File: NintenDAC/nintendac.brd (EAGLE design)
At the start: 42 x 42 mm, 36 parts, among them IC2 REG1117, U1 STM32F10XRXT6, X1 USB-MICROB

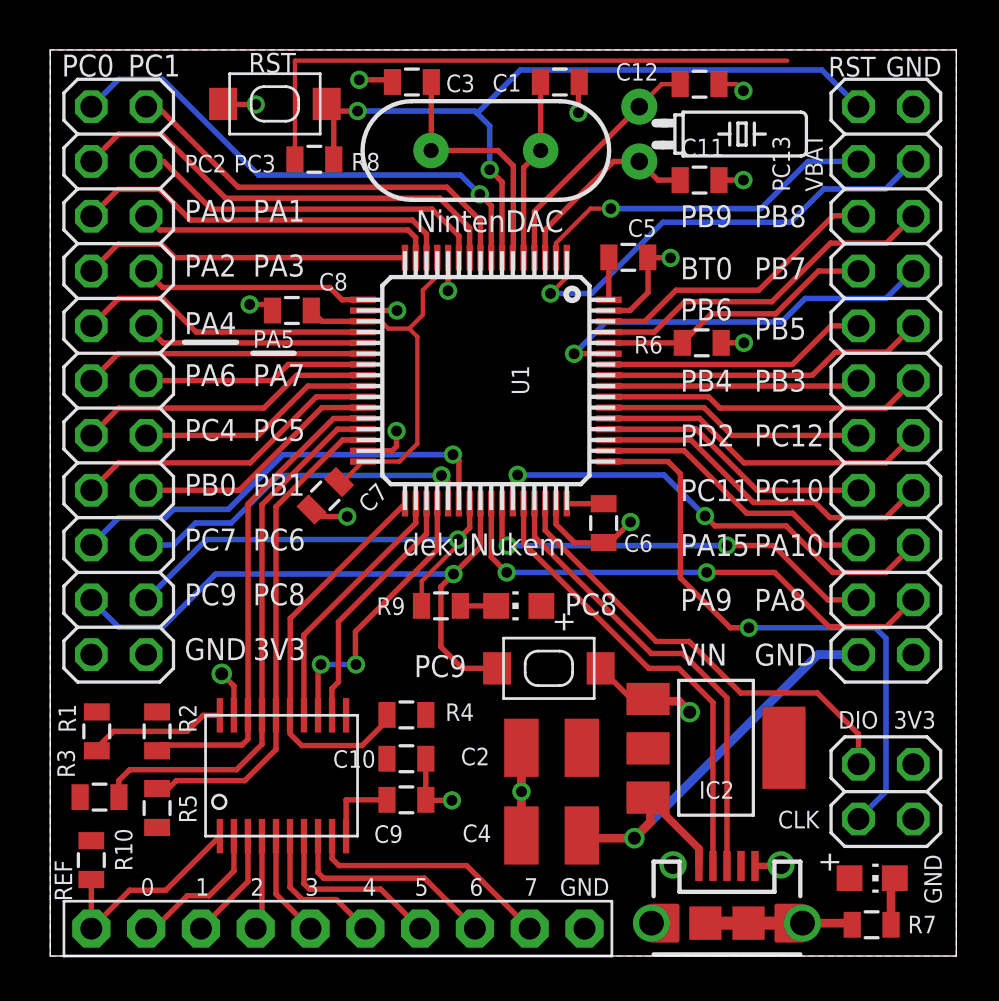
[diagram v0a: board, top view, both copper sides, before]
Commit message: board cleanup
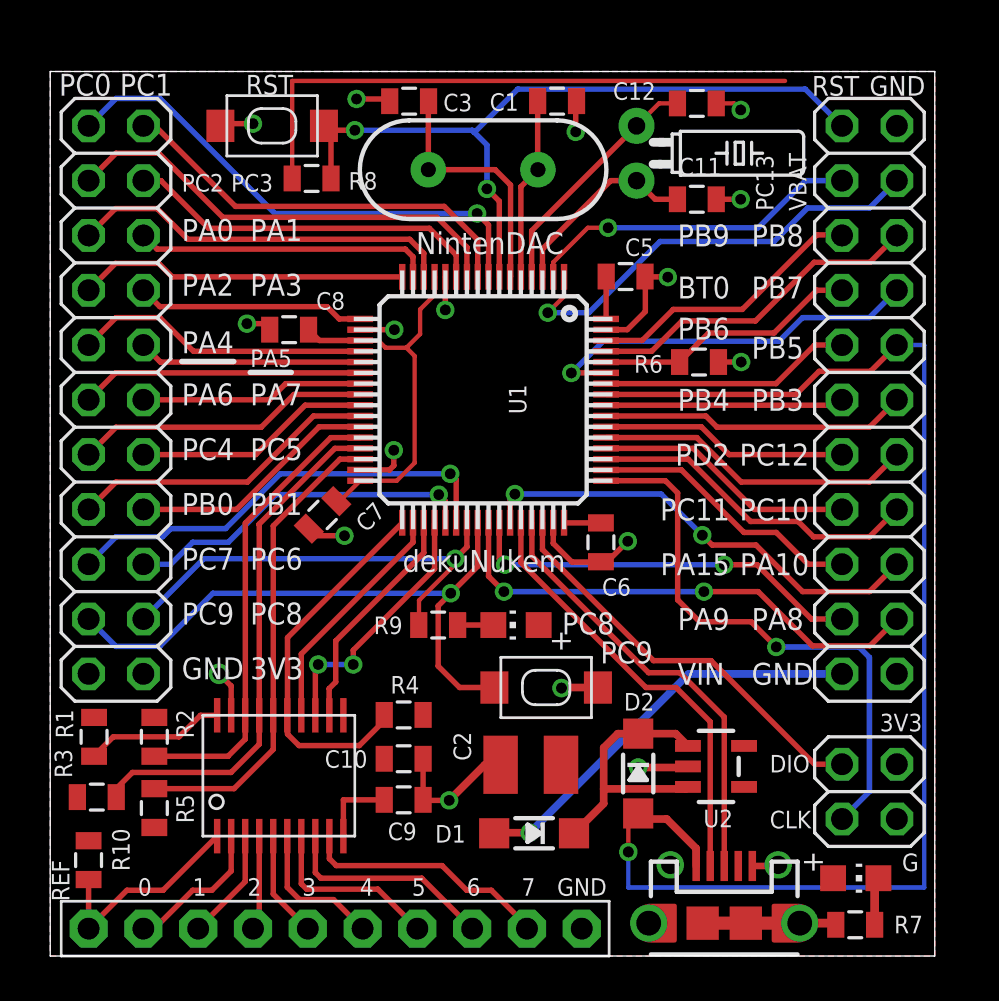
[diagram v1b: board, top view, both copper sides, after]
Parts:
- removed C4: (no value), backplane:C1210
- removed IC2: REG1117, backplane:SOT223
- added D1, D2: (no value), nintendac_mini:SOD-123
- added U2: (no value), nintendac_mini:SOT23-5
- moved C2 1.25 mm to (22.3, 8.86)
- moved JP2 1.17 mm to (38.0, 25.8)
- moved S1 1.02 mm to (10.3, 38.5)
- moved U1 0.90 mm to (20.1, 25.8)
- moved Y1 0.90 mm to (20.1, 36.4)
- moved R8 0.90 mm to (12.1, 36.0)
- moved C11 0.90 mm to (30.0, 35.1)
- moved C12 0.90 mm to (30.0, 39.5)
- moved JP3 0.90 mm to (3.05, 25.8)
- moved Y2 0.90 mm to (27.2, 37.2)
- moved S2 0.90 mm to (23.0, 12.4)
- moved R6 0.90 mm to (30.1, 27.5)
- moved C7 0.90 mm to (12.6, 20.4)
- moved C5 0.90 mm to (26.7, 31.5)
- moved C6 0.90 mm to (25.5, 19.2)
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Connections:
- new net N$2: D1.C, D2.C, U2.1, U2.3
- net +3V3: now also U2.5; no longer IC2.2
- net GND: now also U2.2; no longer C4.2, IC2.1
- net N$58: now also D2.A, X1.VBUS
- net N$66: now also D1.A; no longer C4.1, IC2.3, X1.VBUS
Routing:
- net N$58: track 15.1 -> 62.4 mm, vias 0 -> 1
- net N$2: track 0.00 -> 12.9 mm
- net N$66: track 22.7 -> 19.2 mm
- net GND: track 49.1 -> 46.4 mm
- net N$24: track 21.1 -> 19.2 mm
- net N$22: track 28.0 -> 26.5 mm
- net N$21: track 25.3 -> 24.2 mm
- net N$3: track 21.2 -> 20.4 mm
- net N$19: track 18.3 -> 17.5 mm
- net N$17: track 11.6 -> 10.7 mm
- net N$4: track 21.3 -> 20.5 mm
- net N$18: track 12.0 -> 11.1 mm
- net N$16: track 13.1 -> 12.2 mm
- net N$1: track 36.2 -> 35.4 mm
- net LDAC: track 22.8 -> 22.1 mm
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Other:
- board size 42 x 42 mm -> 41 x 41 mm
- board text added: "G"
